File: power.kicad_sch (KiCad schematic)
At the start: 20 parts, among them U10 TPS7A7001DDA, U8 TLV75733PDBVR

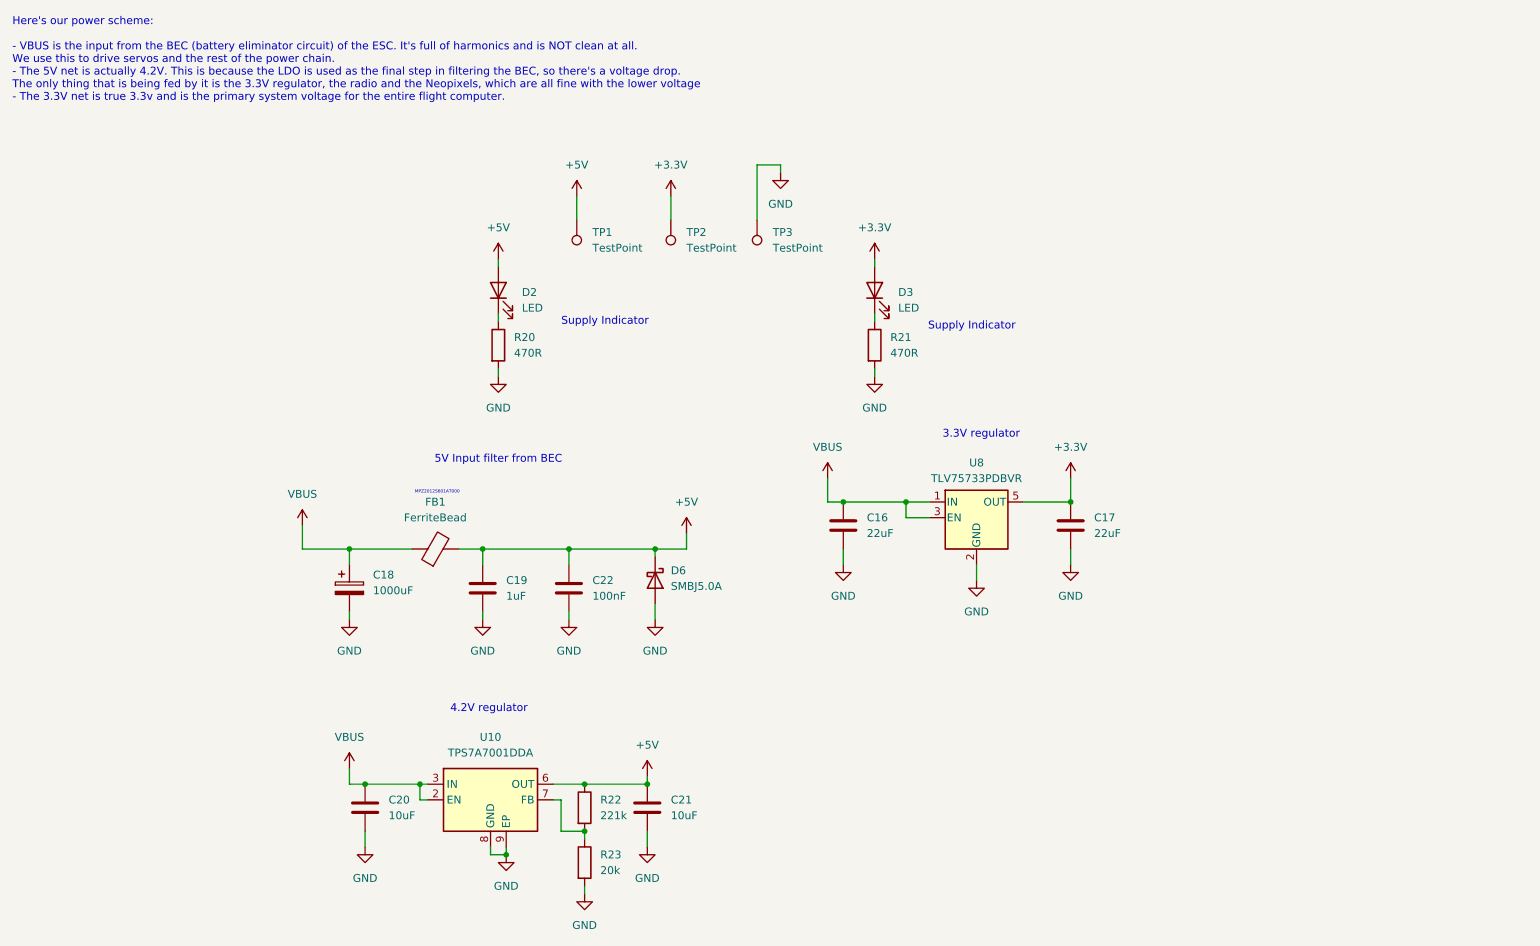
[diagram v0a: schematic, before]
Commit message: Work more on power
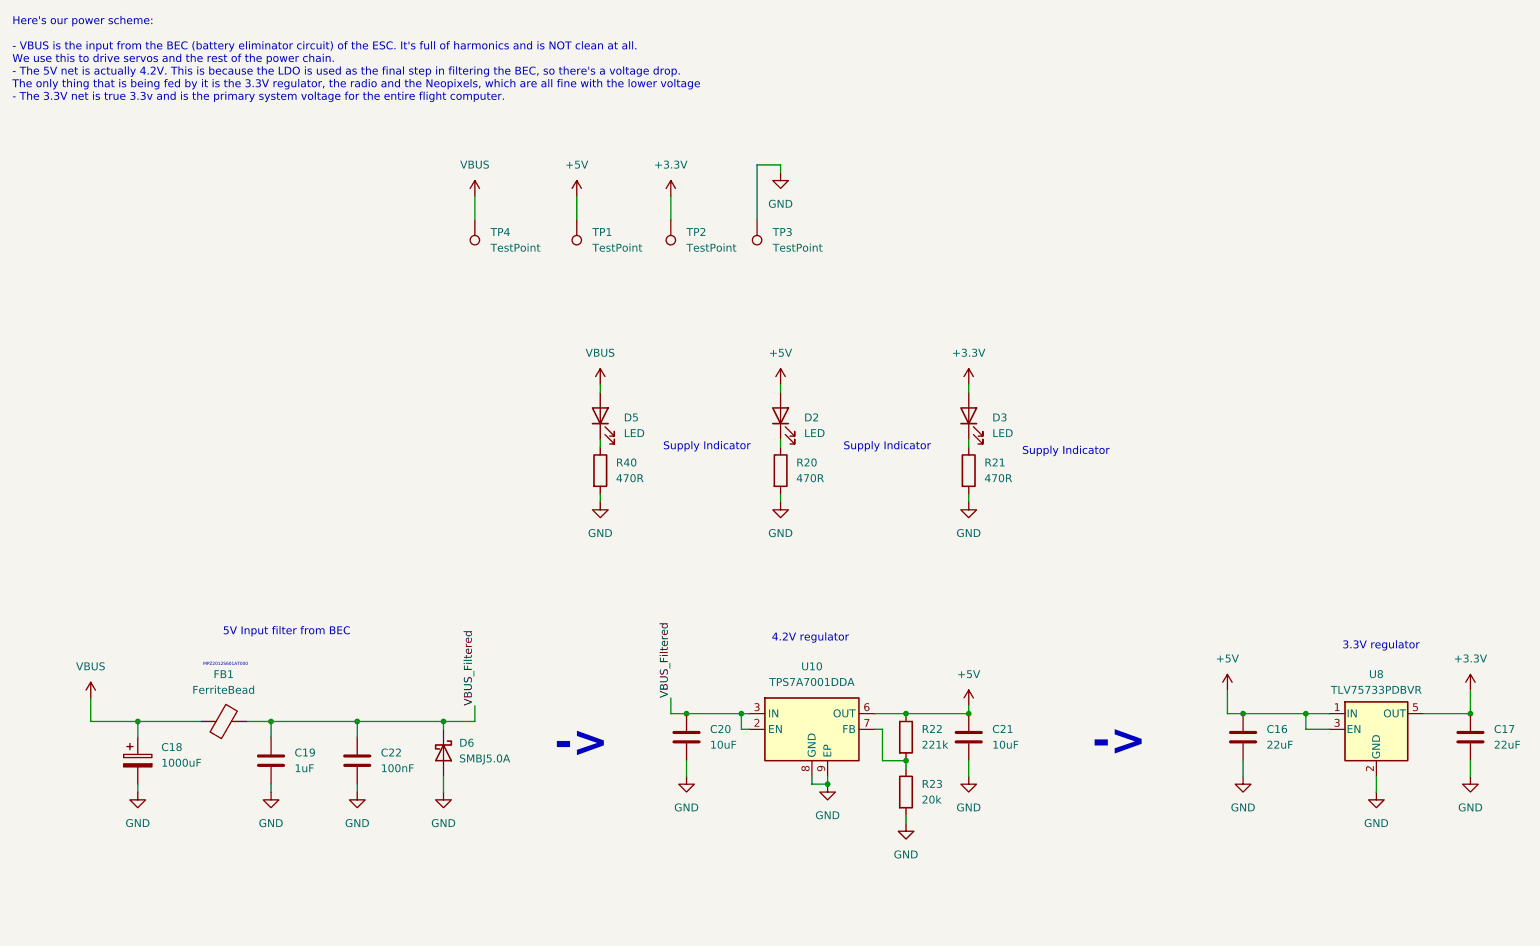
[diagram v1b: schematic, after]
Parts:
- added D5: LED, symbol Device:LED
- added R40: 470R, symbol Device:R
- added TP4: TestPoint, symbol Connector:TestPoint
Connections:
- net +5V: now also C16.1, U8.1 (IN), U8.3 (EN); no longer C19.1, C22.1, D6.1 (K), FB1.2
- net GND: now also R40.2
- net VBUS: now also D5.2 (A), TP4.1; no longer C16.1, C20.1, U10.2 (EN), U10.3 (IN), U8.1 (IN), U8.3 (EN)
- new net: D5.1 (K), R40.1
- new net VBUS_Filtered: C19.1, C20.1, C22.1, D6.1 (K), FB1.2, U10.2 (EN), U10.3 (IN)
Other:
- note added: "->"
- moved on the sheet: C16, C17, C18, C19, C20, C21, C22, D2, D3, D6, FB1, R20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
